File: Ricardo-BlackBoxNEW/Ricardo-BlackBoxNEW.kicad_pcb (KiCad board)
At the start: 4 copper layers, 53.4 x 49.6 mm, 87 parts, among them IC1 XTSD08GLGEAG, IC2 CP2102N-A02-GQFN24, J1 RBUS, J2 USB_C_Receptacle_USB2.0, U1 ESP32-S3, U2 SN65HVD230, U3 LM66200DRLR, U4 MAX77827AEFD+T, U5 SC4215, Y1 40MHz±10ppm

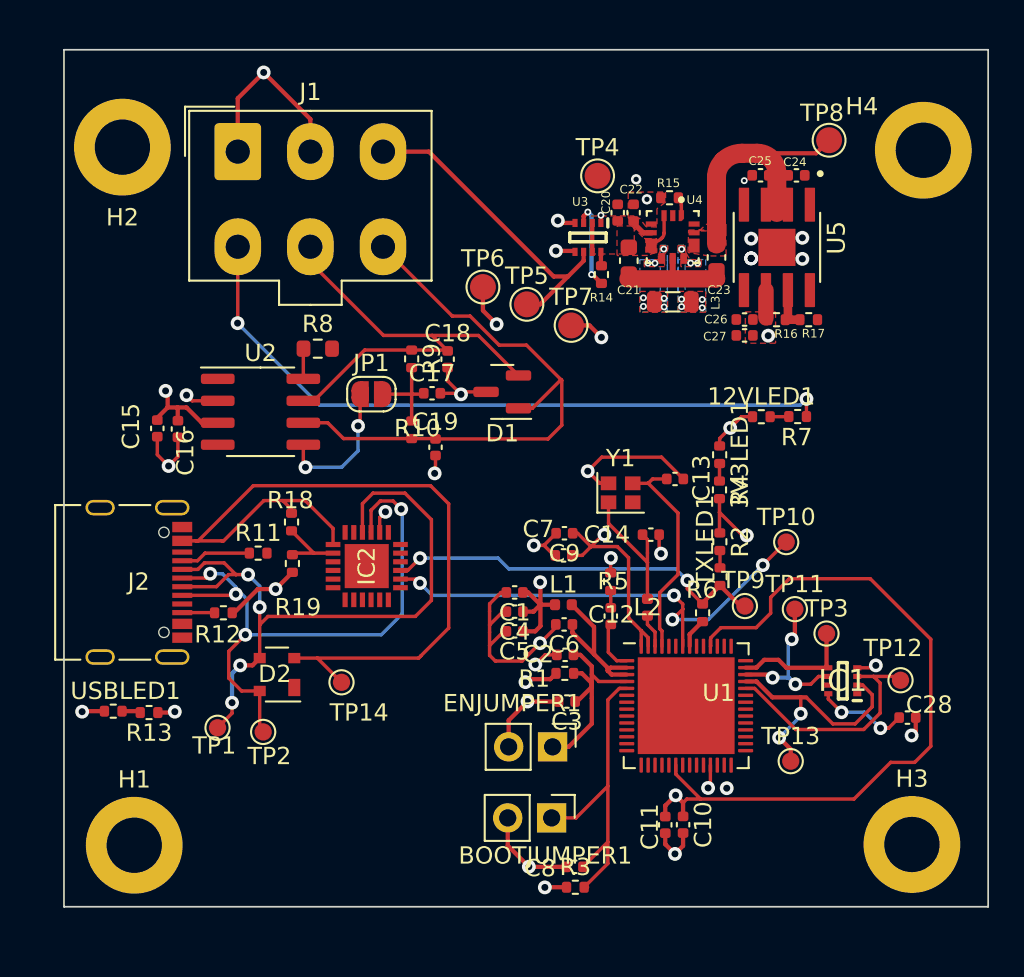
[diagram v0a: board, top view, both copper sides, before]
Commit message: RicardoBlackBox03_06_2023
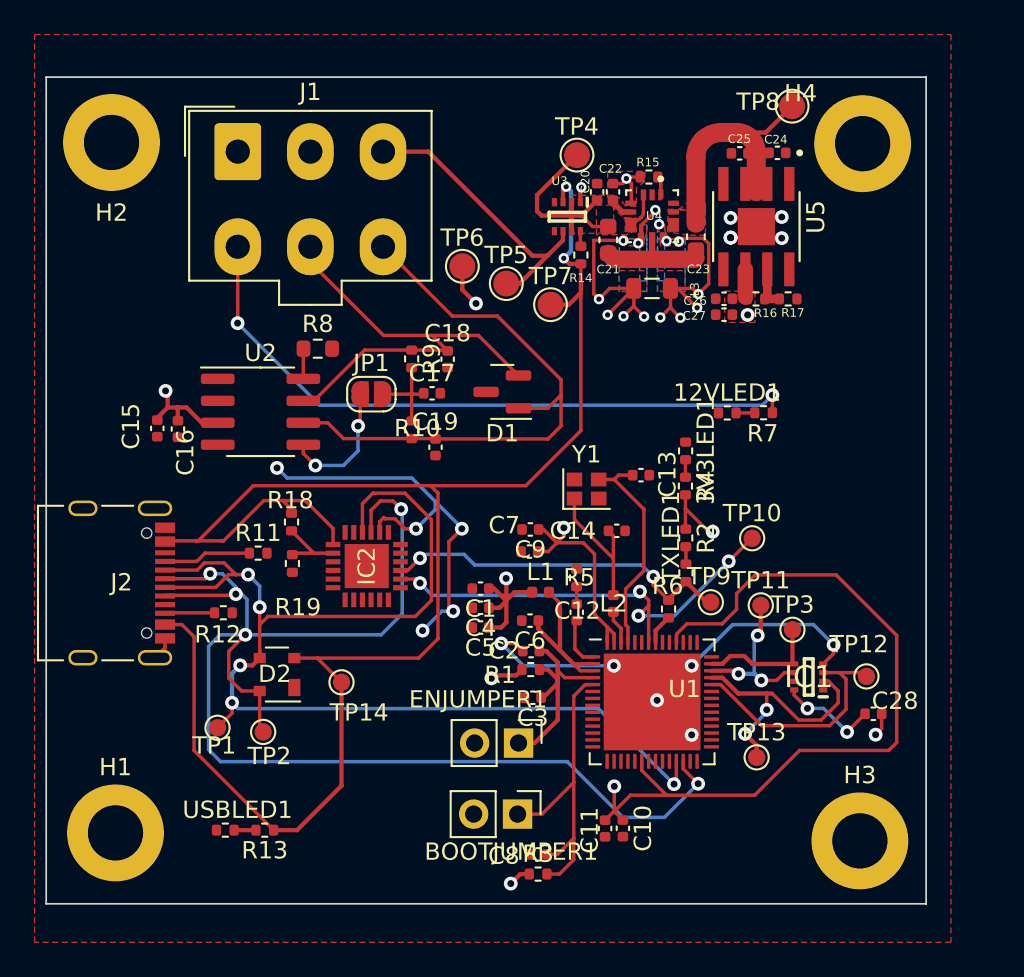
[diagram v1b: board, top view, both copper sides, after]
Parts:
- moved R13 9.54 mm to (131.8, 115.6)
- moved USBLED1 9.45 mm to (129.5, 115.6)
- moved H4 3.53 mm to (166.4, 75.9)
- moved C10 3.49 mm to (152.5, 115.5)
- moved C11 3.49 mm to (151.5, 115.5)
- moved H3 3.02 mm to (166.2, 116.2)
- moved TP8 2.91 mm to (162.3, 73.7)
- moved R3 2.28 mm to (147.6, 118.1)
- moved C8 2.21 mm to (147.6, 117.0)
- moved R4 1.98 mm to (156.1, 95.7)
- moved C13 1.98 mm to (153.6, 95.1)
- moved C3 1.98 mm to (147.3, 107.9)
- moved C9 1.98 mm to (147.2, 98.2)
- moved R7 1.98 mm to (160.7, 91.5)
- moved TP12 1.98 mm to (166.6, 106.7)
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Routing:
- net VBUS: track 55.9 -> 103.3 mm, vias 4 -> 2
- net /Data+: track 37.3 -> 80.1 mm
- net /Data-: track 41.3 -> 71.3 mm
- net GND: track 81.1 -> 66.1 mm, vias 30 -> 18
- net /Power/LX1: track 0.00 -> 14.1 mm
- net /Power/LX2: track 0.00 -> 11.6 mm
- net /Power/BBIN: track 3.68 -> 14.1 mm
- net +3V3: track 82.3 -> 85.7 mm
- net +12V: track 40.5 -> 38.6 mm
- net /TXD: track 22.6 -> 20.7 mm
- net /RXD: track 28.6 -> 26.8 mm
- net RBUS_uC_V: track 18.5 -> 16.8 mm
- net Net-(J2-PadA5): track 4.06 -> 5.07 mm
- net Net-(J2-PadB5): track 1.87 -> 2.88 mm
- net /Power/BBOUT: track 16.7 -> 16.1 mm
- added copper zone on In1.Cu, net +3V3
- added copper zone on In2.Cu, net GND
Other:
- board size 53.4 x 49.6 mm -> 50.9 x 47.8 mm
